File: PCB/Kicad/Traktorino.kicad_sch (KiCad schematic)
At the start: 1 part

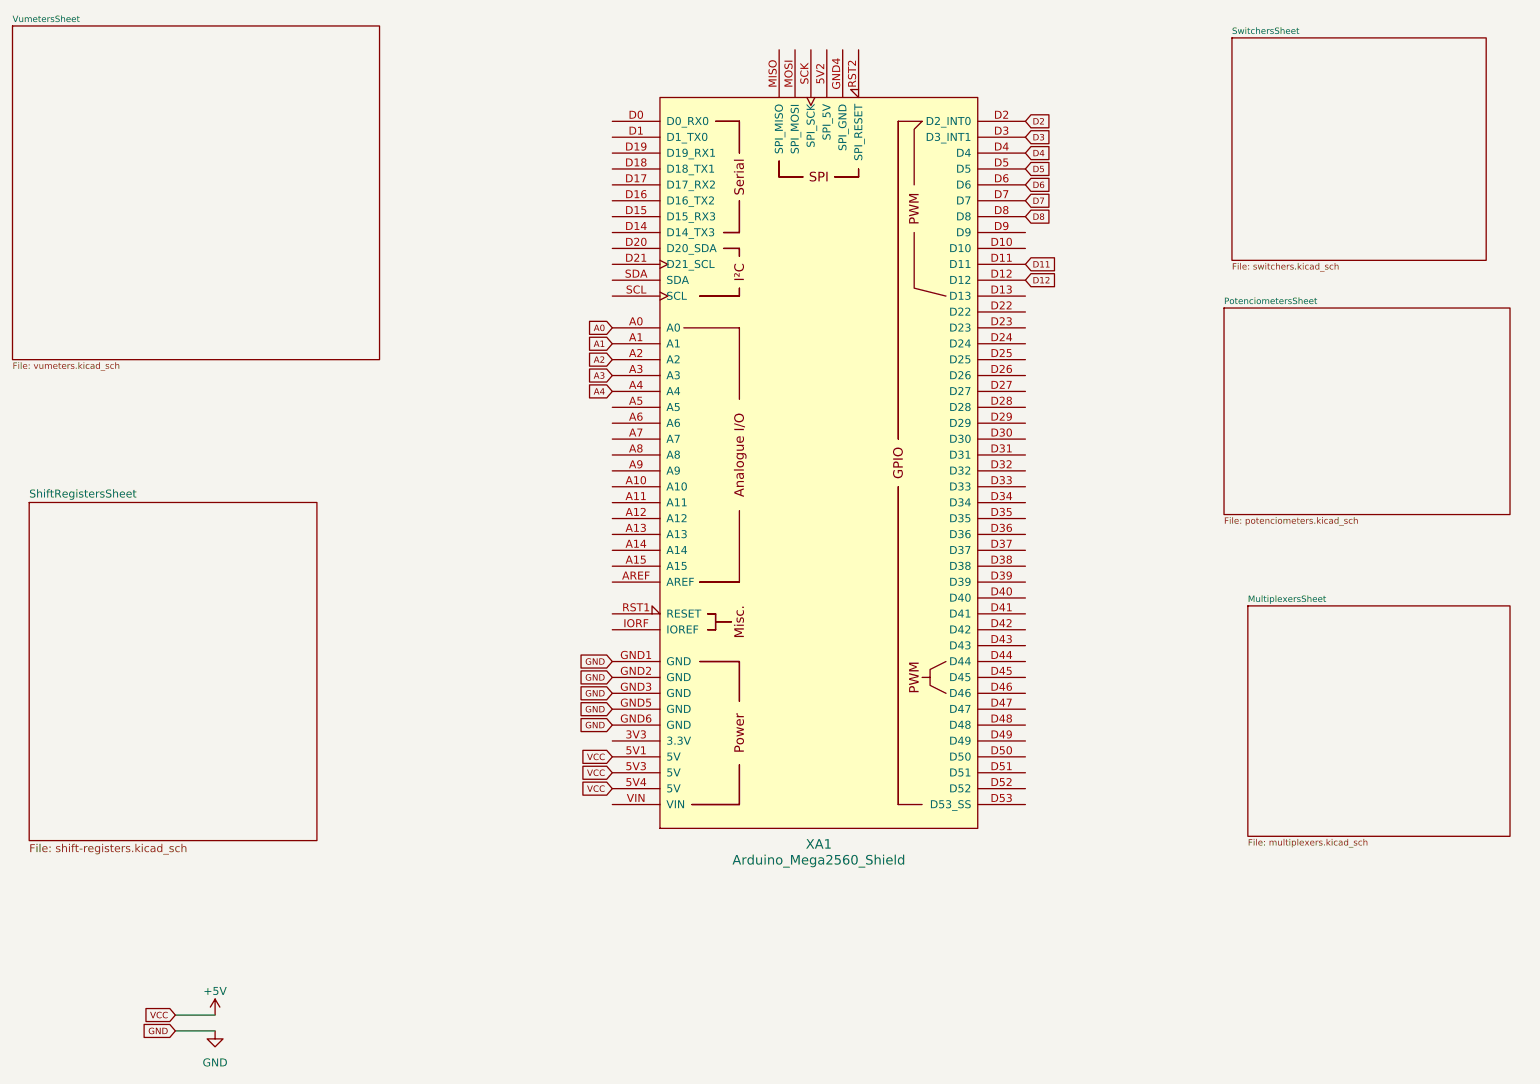
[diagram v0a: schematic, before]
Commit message: trillbar added
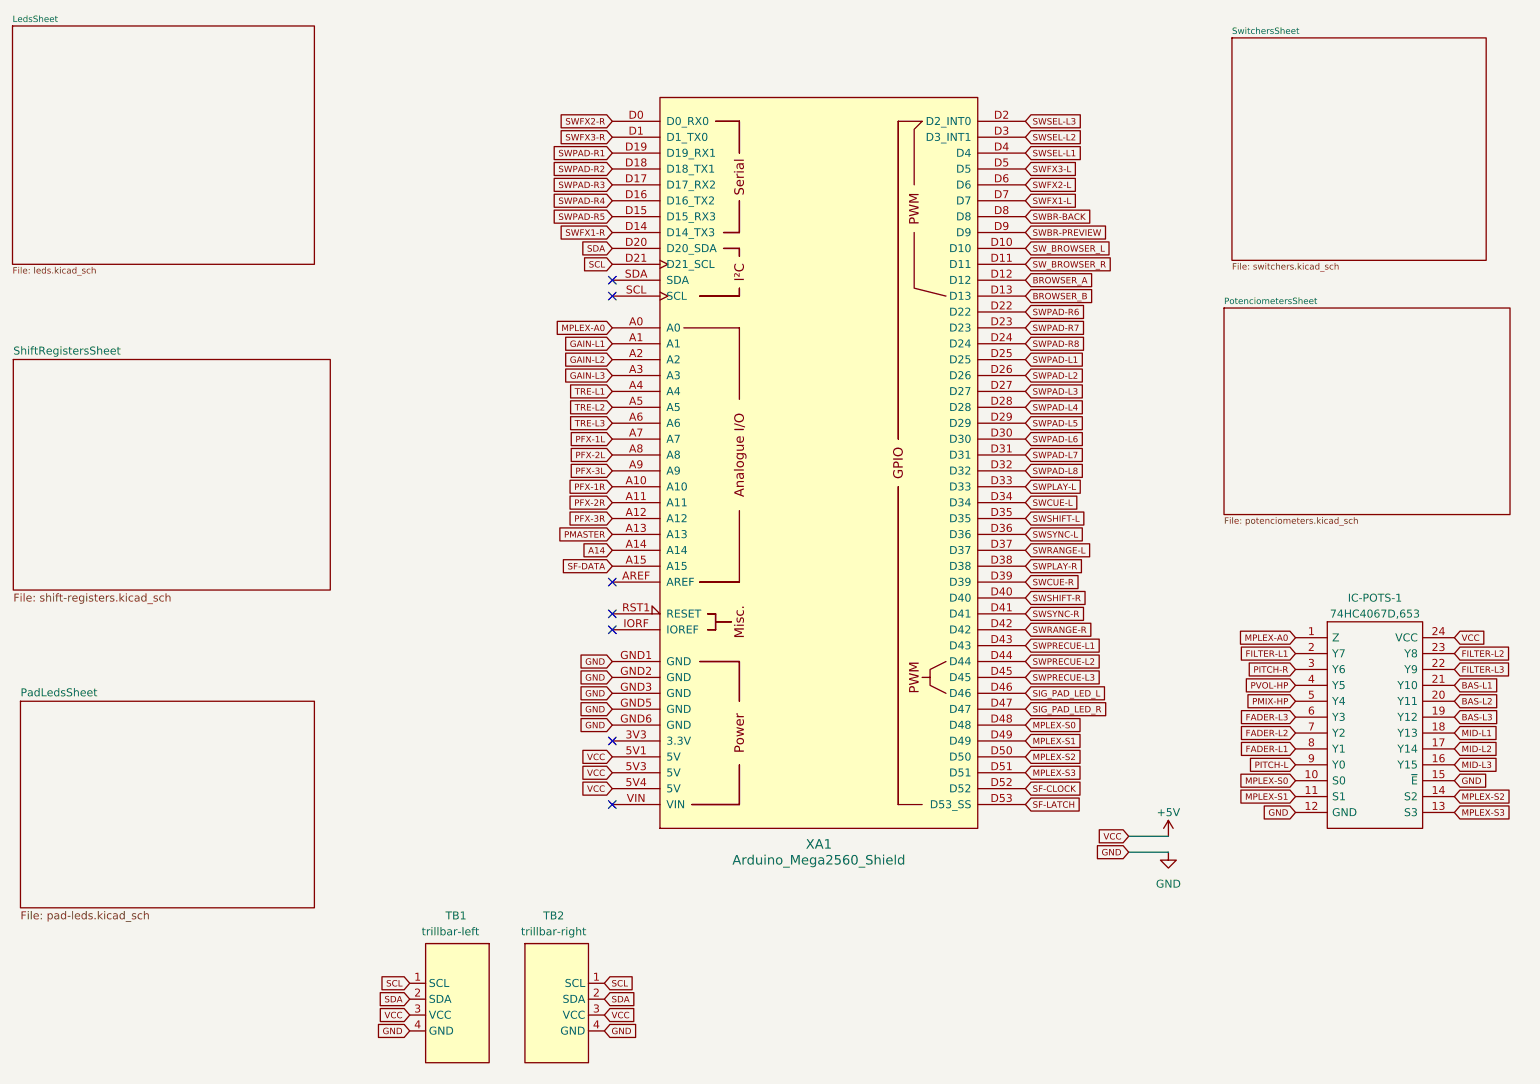
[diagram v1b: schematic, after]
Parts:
- added IC-POTS-1: 74HC4067D,653, Package_SO:SOIC-24W_7.5x15.4mm_P1.27mm, symbol SamacSys_Parts:74HC4067D,653
- added TB1: trillbar-left, Library:trillbar, symbol traktorino-mk2:trillbar
- added TB2: trillbar-right, Library:trillbar, symbol traktorino-mk2:trillbar
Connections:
- net +5V: now also IC-POTS-1.24 (VCC), TB1.3 (VCC), TB2.3 (VCC)
- net GND: now also IC-POTS-1.12 (GND), IC-POTS-1.15 (~E), TB1.4 (GND), TB2.4 (GND)
- net PFX-1R: now reaches XA1.A10
- net PFX-2R: now reaches XA1.A11
- net PFX-3R: now reaches XA1.A12
- net PMASTER: now reaches XA1.A13
- net A14: now reaches XA1.A14
- net SF-DATA: now reaches XA1.A15
- net TRE-L2: now reaches XA1.A5
- net TRE-L3: now reaches XA1.A6
- net PFX-1L: now reaches XA1.A7
- net PFX-2L: now reaches XA1.A8
- net PFX-3L: now reaches XA1.A9
- net SWFX2-R: now reaches XA1.D0 (D0_RX0)
- net SWFX3-R: now reaches XA1.D1 (D1_TX0)
- net SW_BROWSER_L: now reaches XA1.D10
- net BROWSER_B: now reaches XA1.D13
- net SWFX1-R: now reaches XA1.D14 (D14_TX3)
- net SWPAD-R5: now reaches XA1.D15 (D15_RX3)
- net SWPAD-R4: now reaches XA1.D16 (D16_TX2)
- net SWPAD-R3: now reaches XA1.D17 (D17_RX2)
- net SWPAD-R2: now reaches XA1.D18 (D18_TX1)
- net SWPAD-R1: now reaches XA1.D19 (D19_RX1)
- net SDA: now reaches XA1.D20 (D20_SDA)
- net SDA: now also TB1.2 (SDA), TB2.2 (SDA)
- net SCL: now reaches XA1.D21 (D21_SCL)
- net SCL: now also TB1.1 (SCL), TB2.1 (SCL)
- net SWPAD-R6: now reaches XA1.D22
- net SWPAD-R7: now reaches XA1.D23
- net SWPAD-R8: now reaches XA1.D24
- net SWPAD-L1: now reaches XA1.D25
- net SWPAD-L2: now reaches XA1.D26
- net SWPAD-L3: now reaches XA1.D27
- net SWPAD-L4: now reaches XA1.D28
- net SWPAD-L5: now reaches XA1.D29
- net SWPAD-L6: now reaches XA1.D30
- net SWPAD-L7: now reaches XA1.D31
- net SWPAD-L8: now reaches XA1.D32
- net SWPLAY-L: now reaches XA1.D33
- net SWCUE-L: now reaches XA1.D34
- net SWSHIFT-L: now reaches XA1.D35
- net SWSYNC-L: now reaches XA1.D36
- net SWRANGE-L: now reaches XA1.D37
- net SWPLAY-R: now reaches XA1.D38
- net SWCUE-R: now reaches XA1.D39
- net SWSHIFT-R: now reaches XA1.D40
- net SWSYNC-R: now reaches XA1.D41
- net SWRANGE-R: now reaches XA1.D42
- net SWPRECUE-L1: now reaches XA1.D43
- net SWPRECUE-L2: now reaches XA1.D44
- net SWPRECUE-L3: now reaches XA1.D45
- net SIG_PAD_LED_L: now reaches XA1.D46
- net SIG_PAD_LED_R: now reaches XA1.D47
- net MPLEX-S0: now reaches XA1.D48
- net MPLEX-S0: now also IC-POTS-1.10 (S0)
- net MPLEX-S1: now reaches XA1.D49
- net MPLEX-S1: now also IC-POTS-1.11 (S1)
- net MPLEX-S2: now reaches XA1.D50
- net MPLEX-S2: now also IC-POTS-1.14 (S2)
- net MPLEX-S3: now reaches XA1.D51
- net MPLEX-S3: now also IC-POTS-1.13 (S3)
- net SF-CLOCK: now reaches XA1.D52
- net SF-LATCH: now reaches XA1.D53 (D53_SS)
- net SWBR-PREVIEW: now reaches XA1.D9
- net A0 renamed MPLEX-A0
- net MPLEX-A0: now also IC-POTS-1.1 (Z)
- net A1 renamed GAIN-L1
- net A2 renamed GAIN-L2
- net A3 renamed GAIN-L3
- net A4 renamed TRE-L1
- net D11 renamed SW_BROWSER_R
- net D12 renamed BROWSER_A
- net D2 renamed SWSEL-L3
- net D3 renamed SWSEL-L2
- net D4 renamed SWSEL-L1
- net D5 renamed SWFX3-L
- net D6 renamed SWFX2-L
- net D7 renamed SWFX1-L
- net D8 renamed SWBR-BACK
- new net BAS-L1: IC-POTS-1.21 (Y10)
- new net BAS-L2: IC-POTS-1.20 (Y11)
- new net BAS-L3: IC-POTS-1.19 (Y12)
- new net FADER-L1: IC-POTS-1.8 (Y1)
- new net FADER-L2: IC-POTS-1.7 (Y2)
- new net FADER-L3: IC-POTS-1.6 (Y3)
- new net FILTER-L1: IC-POTS-1.2 (Y7)
- new net FILTER-L2: IC-POTS-1.23 (Y8)
- new net FILTER-L3: IC-POTS-1.22 (Y9)
- new net MID-L1: IC-POTS-1.18 (Y13)
- new net MID-L2: IC-POTS-1.17 (Y14)
- new net MID-L3: IC-POTS-1.16 (Y15)
- new net PITCH-L: IC-POTS-1.9 (Y0)
- new net PITCH-R: IC-POTS-1.3 (Y6)
- new net PMIX-HP: IC-POTS-1.5 (Y4)
- new net PVOL-HP: IC-POTS-1.4 (Y5)
- no-connect marks 0 -> 7
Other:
- sheet VumetersSheet renamed LedsSheet
- removed sheet MultiplexersSheet
- added sheet PadLedsSheet (pad-leds.kicad_sch)
- sheet LedsSheet: file vumeters.kicad_sch -> leds.kicad_sch
